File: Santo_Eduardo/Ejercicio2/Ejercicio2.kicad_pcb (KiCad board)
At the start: 2 copper layers, 40.6 x 61 mm, 15 parts, among them J1 DB9, U1 AMIS42665TJAA1RG, U2 MAX232

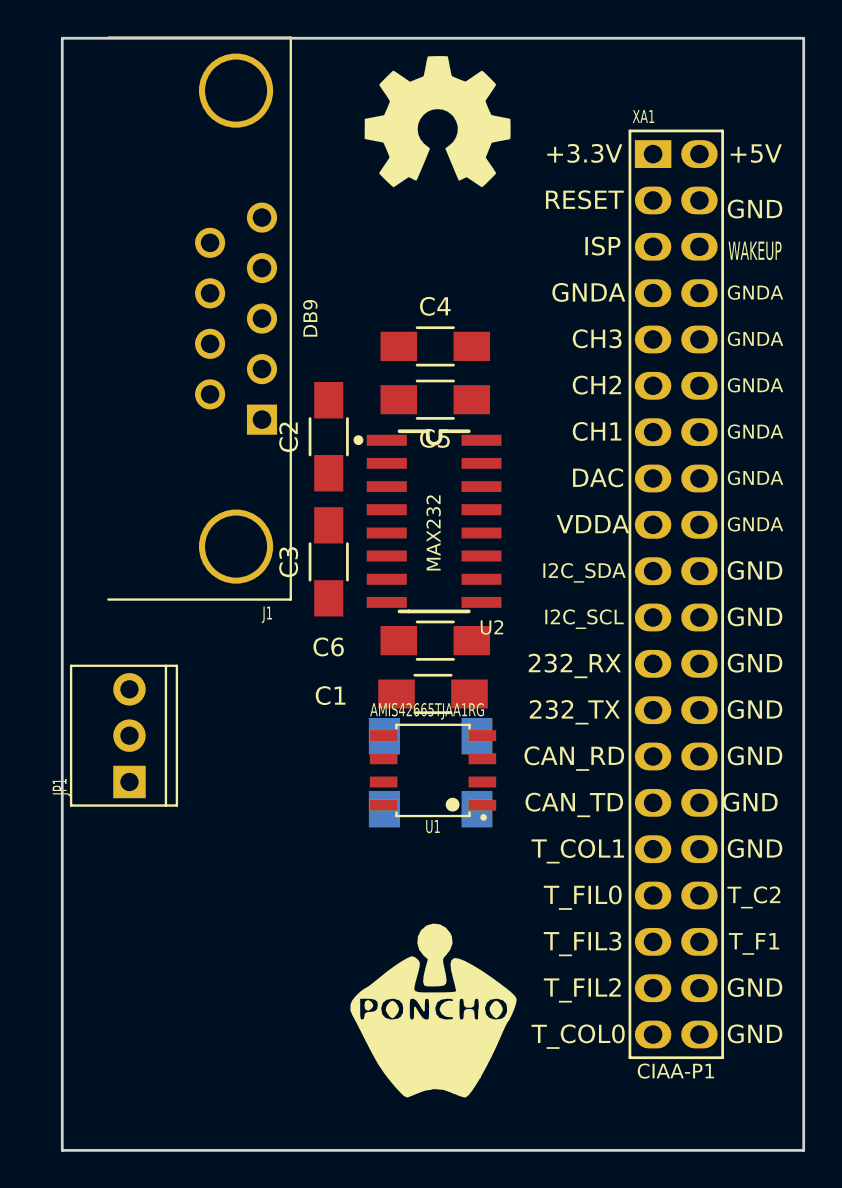
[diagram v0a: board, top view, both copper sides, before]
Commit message: Minor changes on pcb
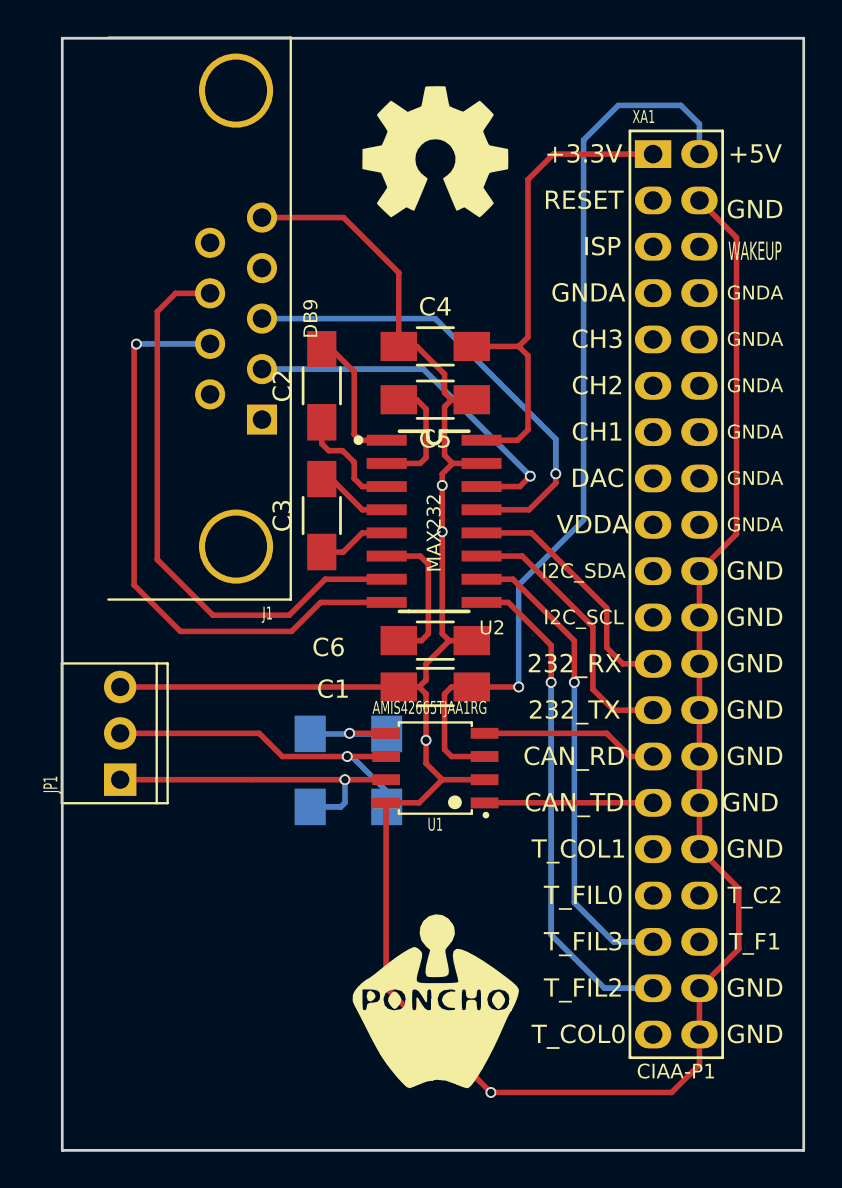
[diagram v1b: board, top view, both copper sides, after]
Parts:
- moved R2 4.95 mm to (156.2, 61.1)
- moved R1 4.07 mm to (152.0, 61.1)
- moved C2 2.82 mm to (152.7, 40.0)
- moved C3 2.57 mm to (152.7, 47.1)
- moved G101 1.66 mm to (158.9, 27.2)
- moved JP1 0.52 mm to (141.6, 59.1)
- moved G*** 0.52 mm to (158.9, 73.8)
- moved C1 0.40 mm to (158.9, 56.5)
- moved U1 0.18 mm to (158.9, 61.0)
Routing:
- net GND: track 0.00 -> 147.7 mm, vias 0 -> 4
- net +5V: track 0.00 -> 50.3 mm, vias 0 -> 1
- net Net-(J1-Pad7): track 0.00 -> 32.9 mm, vias 0 -> 1
- net Net-(J1-Pad8): track 0.00 -> 31.6 mm
- net /Conector y CAN/RTS: track 0.00 -> 27.5 mm, vias 0 -> 1
- net +3.3V: track 0.00 -> 26.9 mm
- net /Conector y CAN/CTS: track 0.00 -> 26.0 mm, vias 0 -> 1
- net Net-(J1-Pad3): track 0.00 -> 25.9 mm, vias 0 -> 1
- net Net-(J1-Pad2): track 0.00 -> 20.0 mm, vias 0 -> 1
- net /Conector y CAN/CAN_L: track 0.00 -> 18.9 mm, vias 0 -> 1
- net /Conector y CAN/CAN_H: track 0.00 -> 17.8 mm, vias 0 -> 1
- net /Conector y CAN/RXD: track 0.00 -> 14.9 mm
- net /Conector y CAN/TXD: track 0.00 -> 13.6 mm
- net /Conector y CAN/CANRX: track 0.00 -> 9.76 mm
- net /Conector y CAN/CANTX: track 0.00 -> 9.24 mm
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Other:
- net class Default: clearance 0.2 -> 0.3048; trace_width 0.25 -> 0.3048
- rule trace_clearance: 0.2 -> 0.3048
